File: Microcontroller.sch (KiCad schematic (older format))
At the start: 32 parts, among them J3 USB_B, J4 SWD, J5 DEBUG, Q1 BC817, U3 STM32F401VETx, U4 USBUF02W6, Y1 8MHz

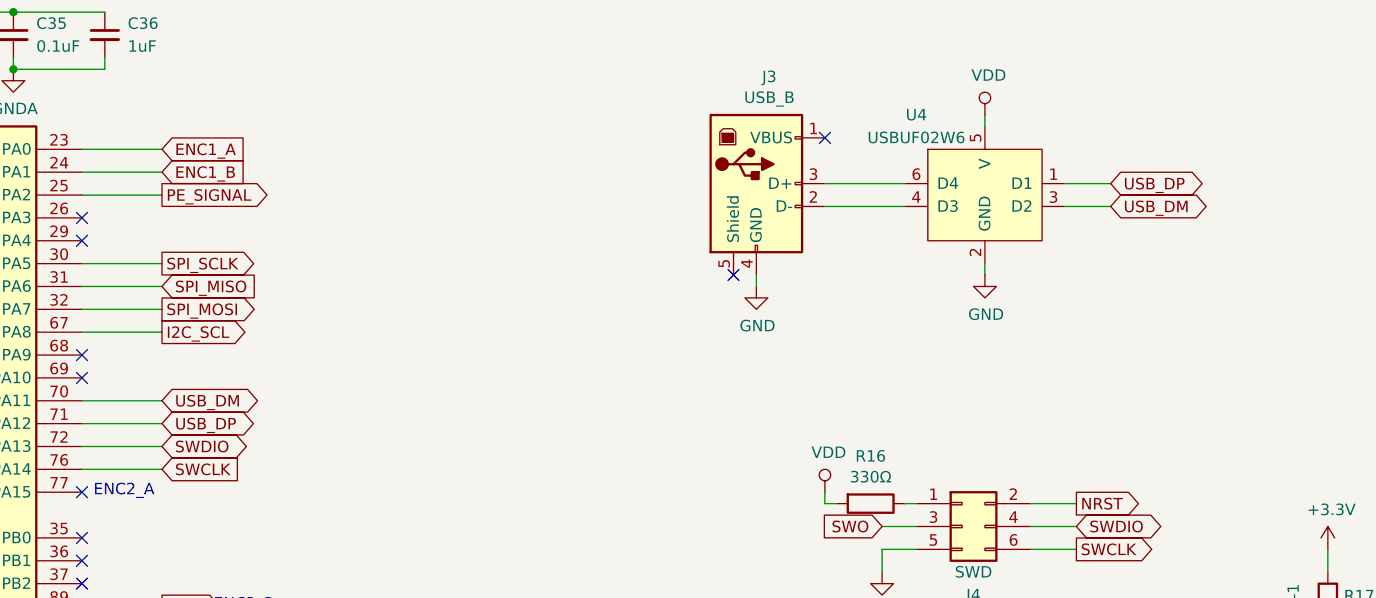
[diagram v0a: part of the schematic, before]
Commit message: Update USBUF02W6
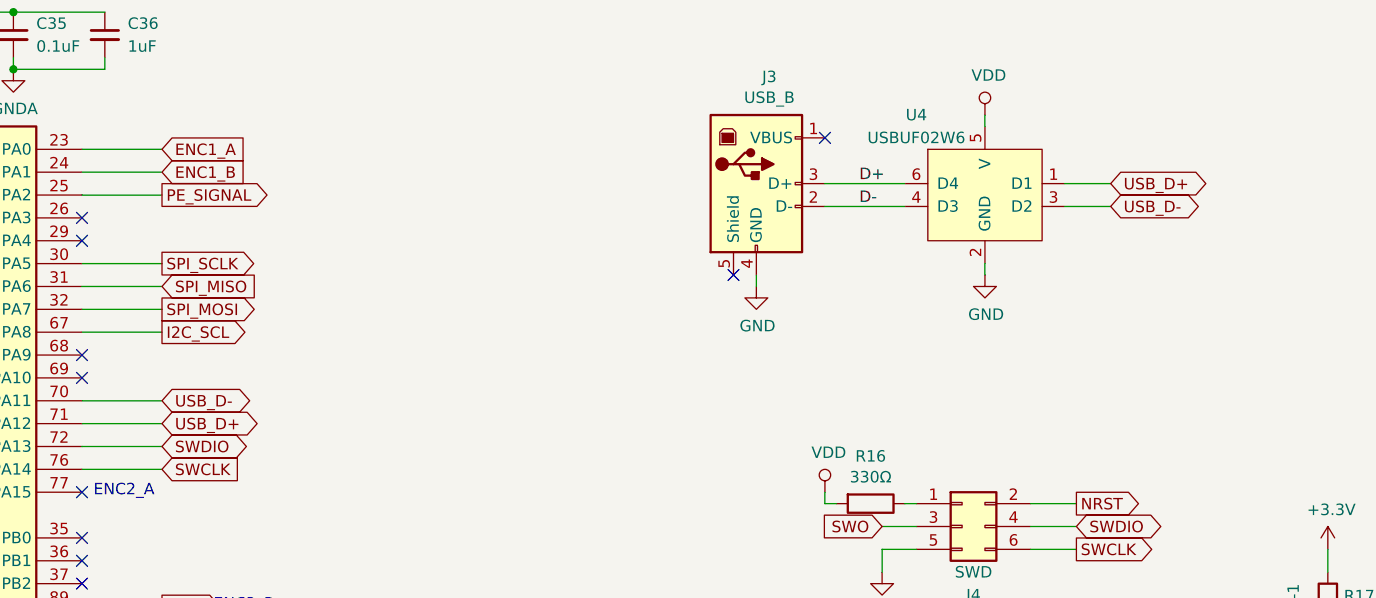
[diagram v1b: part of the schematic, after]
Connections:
- net D-: now reaches J3.2 (D-), U4.4 (D3)
- net D+: now reaches J3.3 (D+), U4.6 (D4)
- net USB_DM renamed USB_D-
- net USB_DP renamed USB_D+
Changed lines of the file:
@@
 	4650 3950 5000 3950
 Text GLabel 5000 2750 2    50   BiDi ~ 0
-USB_DP
-Text GLabel 5000 2650 2    50   BiDi ~ 0
-USB_DM
+USB_D+
 Wire Wire Line
 	4650 2650 5000 2650
@@
 	8600 1400 8600 1450
 Text GLabel 9150 1800 2    50   BiDi ~ 0
-USB_DM
+USB_D-
 Text GLabel 9150 1700 2    50   BiDi ~ 0
-USB_DP
+USB_D+
 Wire Wire Line
 	8950 1700 9150 1700
@@
 Wire Wire Line
 	2750 2050 2750 2250
+Text Label 8050 1700 0    50   ~ 0
+D+
+Text Label 8050 1800 0    50   ~ 0
+D-
+Text GLabel 5000 2650 2    50   BiDi ~ 0
+USB_D-
 $EndSCHEMATC
